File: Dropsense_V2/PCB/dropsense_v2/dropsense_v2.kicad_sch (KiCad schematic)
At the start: 28 parts, among them J1 Micro_SD_Card_Det_Hirose_DM3AT, J2 USB_B_Micro, J3 battery socket, SW1 SW_Push, SW2 SW_Push, U1 ESP32-S3-WROOM-1, U2 MPU-6050, U3 TP4056-42-ESOP8, U4 ME6211C10M5

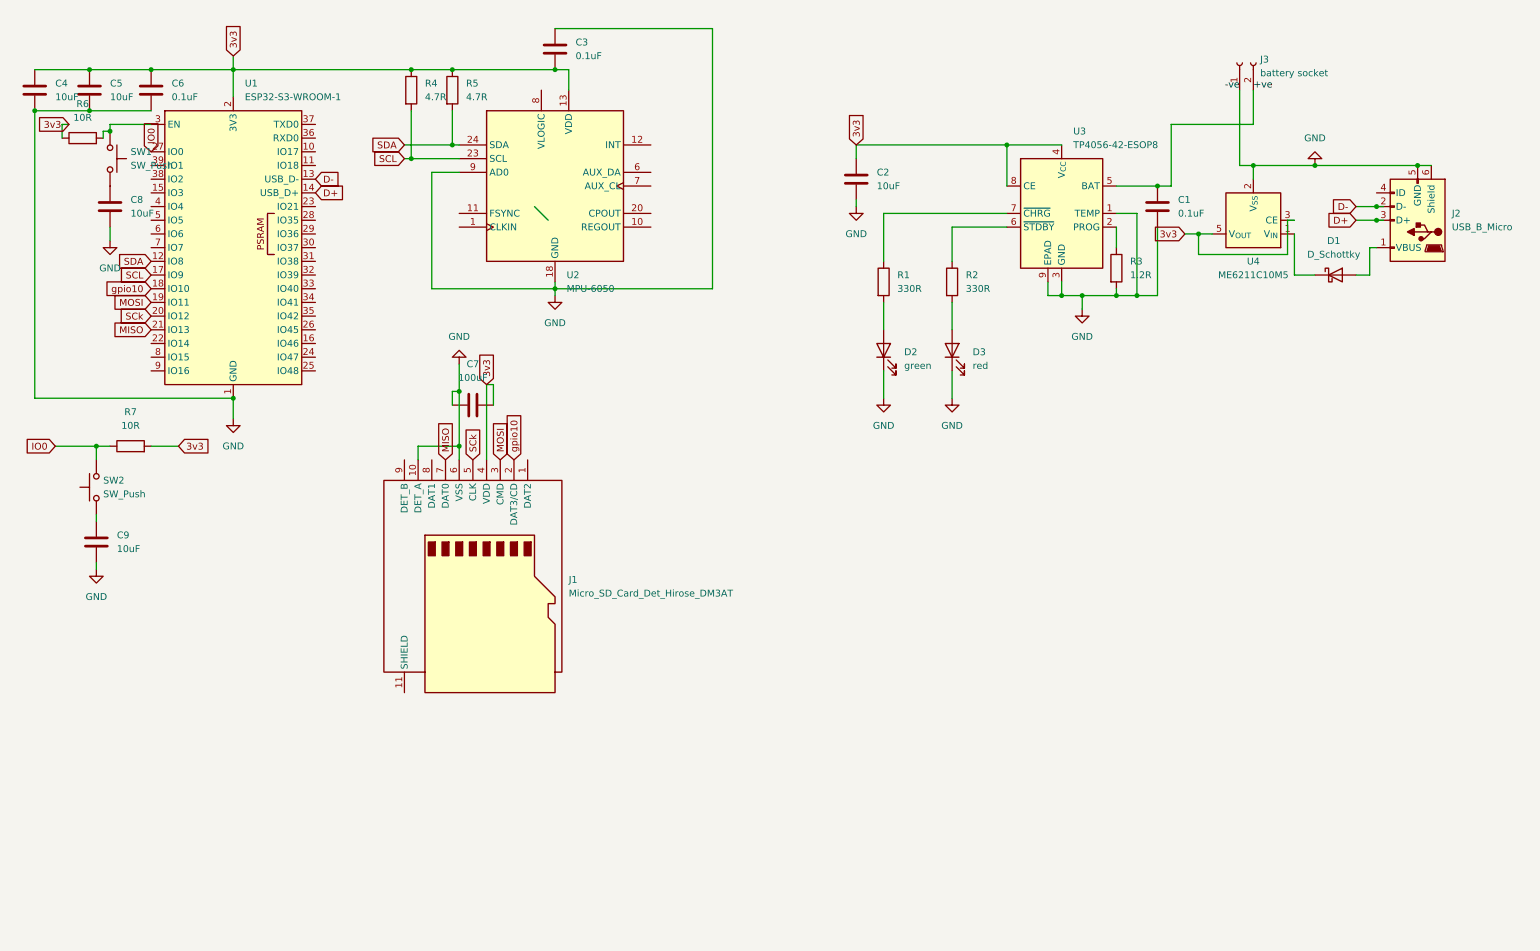
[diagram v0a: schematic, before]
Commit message: STARTED DROPSENSE V2!!!!!!
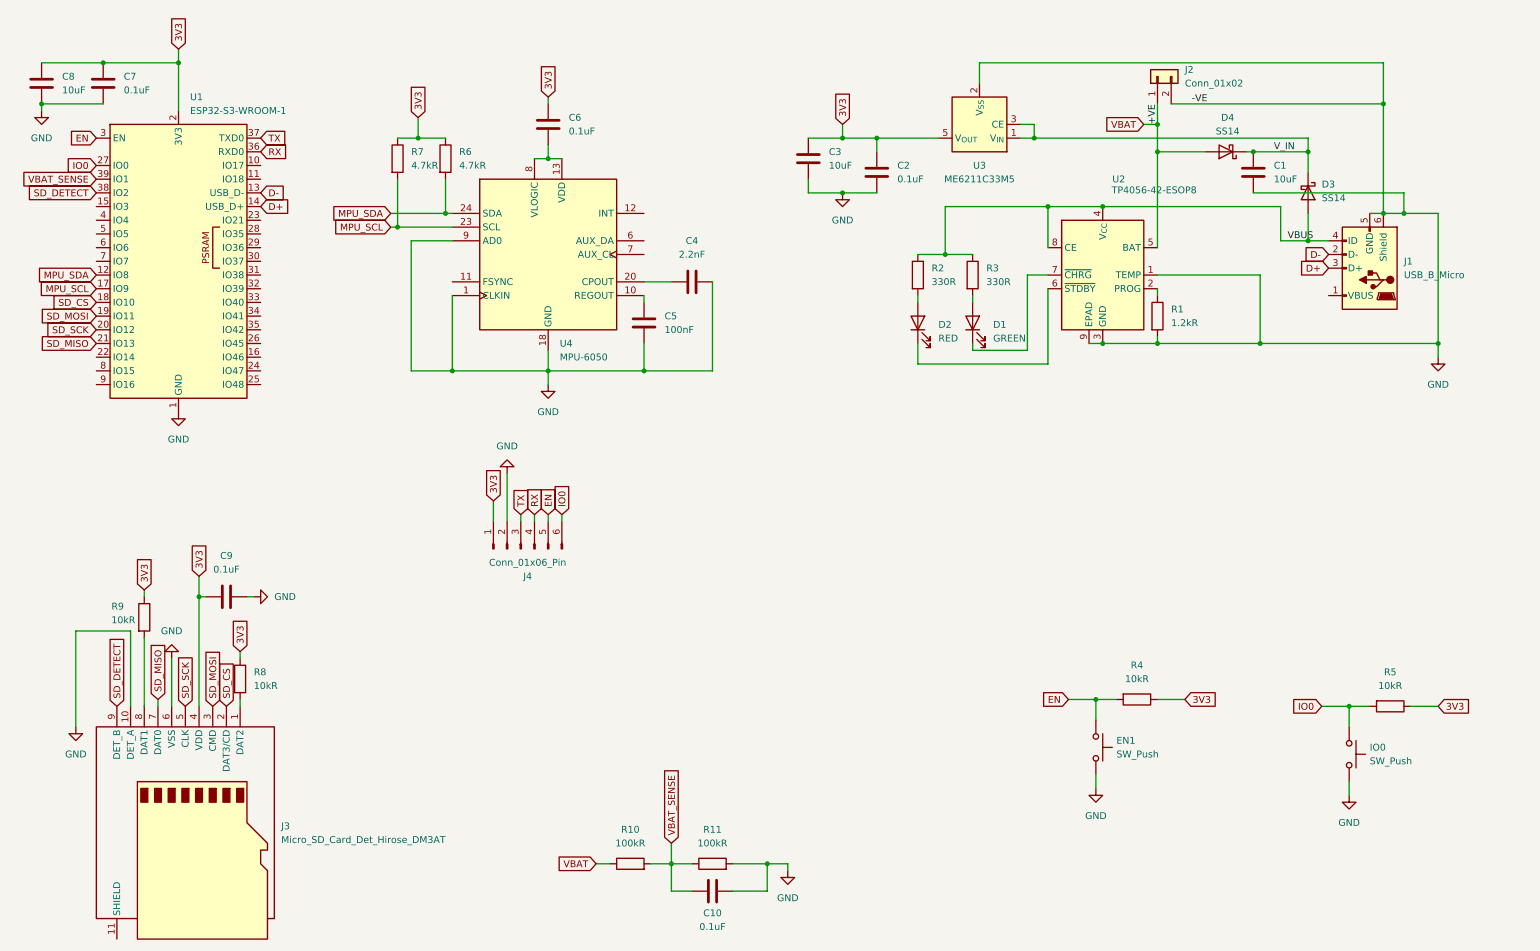
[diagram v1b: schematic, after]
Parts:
- removed D1: D_Schottky, Diode_SMD:D_0805_2012Metric, symbol Device:D_Schottky
- removed D3: red, LED_SMD:LED_0805_2012Metric, symbol Device:LED
- removed J1: Micro_SD_Card_Det_Hirose_DM3AT, Connector_Card:microSD_HC_Hirose_DM3AT-SF-PEJM5, symbol Connector:Micro_SD_Card_Det_Hirose_DM3AT
- removed J2: USB_B_Micro, Connector_USB:USB_Micro-B_Amphenol_10103594-0001LF_Horizontal, symbol Connector:USB_B_Micro
- removed J3: battery socket, Connector_JST:JST_PH_B2B-PH-K_1x02_P2.00mm_Vertical, symbol Connector:Conn_01x02_Socket
- removed SW1, SW2: SW_Push, Button_Switch_THT:SW_PUSH_6mm_H4.3mm, symbol Switch:SW_Push
- removed U2: MPU-6050, Sensor_Motion:InvenSense_QFN-24_4x4mm_P0.5mm, symbol Sensor_Motion:MPU-6050
- removed U3: TP4056-42-ESOP8, Package_SO:SOIC-8-1EP_3.9x4.9mm_P1.27mm_EP2.41x3.3mm_ThermalVias, symbol Battery_Management:TP4056-42-ESOP8
- removed U4: ME6211C10M5, Package_TO_SOT_SMD:SOT-23-5, symbol Regulator_Linear:ME6211C10M5
- added C10: 0.1uF, Capacitor_SMD:C_0805_2012Metric, symbol Device:C
- added D1: GREEN, LED_SMD:LED_0805_2012Metric, symbol Device:LED
- added D3, D4: SS14, Diode_SMD:D_SMA, symbol Diode:SS14
- added EN1, IO0: SW_Push, Button_Switch_SMD:SW_Push_1P1T-SH_NO_CK_KMR2xxG, symbol Switch:SW_Push
- added J1: USB_B_Micro, Connector_USB:USB_Micro-B_Molex-105017-0001, symbol Connector:USB_B_Micro
- added J2: Conn_01x02, Connector_JST:JST_XH_B2B-XH-A_1x02_P2.50mm_Vertical, symbol Connector_Generic:Conn_01x02
- added J3: Micro_SD_Card_Det_Hirose_DM3AT, Connector_Card:microSD_HC_Hirose_DM3AT-SF-PEJM5, symbol Connector:Micro_SD_Card_Det_Hirose_DM3AT
- added J4: Conn_01x06_Pin, Connector_PinHeader_2.54mm:PinHeader_1x06_P2.54mm_Vertical, symbol Connector:Conn_01x06_Pin
- added R10, R11: 100kR, Resistor_SMD:R_0805_2012Metric, symbol Device:R
- added R8, R9: 10kR, Resistor_SMD:R_0805_2012Metric, symbol Device:R
- added U2: TP4056-42-ESOP8, Package_SO:SOIC-8-1EP_3.9x4.9mm_P1.27mm_EP2.41x3.3mm_ThermalVias, symbol Battery_Management:TP4056-42-ESOP8
- added U3: ME6211C33M5, Package_TO_SOT_SMD:SOT-23-5, symbol Regulator_Linear:ME6211C33M5
- added U4: MPU-6050, Sensor_Motion:InvenSense_QFN-24_4x4mm_P0.5mm, symbol Sensor_Motion:MPU-6050
- C1, C3: value 0.1uF -> 10uF
- C2, C9: value 10uF -> 0.1uF
- C4: value 10uF -> 2.2nF
- C5: value 10uF -> 100nF
- C7: value 100uF -> 0.1uF
- D2: value green -> RED
- R1: value 330R -> 1.2kR
- R3: value 1.2R -> 330R
- R4, R5: value 4.7R -> 10kR
- R6, R7: value 10R -> 4.7kR
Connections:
- net D+: now also J1.3 (D+)
- net D-: now also J1.2 (D-)
- net GND: now also C3.2, C5.1, C7.2, R1.2, C10.2, EN1.2, IO0.2, J1.5 (GND), J1.6 (Shield), J2.2 (Pin_2), J3.10 (DET_A), J3.6 (VSS), J4.2 (Pin_2), R11.2, U2.1 (TEMP), U2.3 (GND), U2.9 (EPAD), U3.2 (V_{SS}), U4.1 (CLKIN), U4.18 (GND), U4.9 (AD0); no longer C3.1, C5.2, C6.2, C7.1, D2.1 (K), R3.2
- net IO0: now also R5.2, IO0.1, J4.6 (Pin_6); no longer R7.1
- net at R2.2: now also D2.2 (A)
- net 3V3: now reaches C9.1
- net 3V3: now also C2.1, C3.1, C6.1, C7.1, C8.1, R4.1, R5.1, R6.1, R7.1, U1.2 (3V3), J3.4 (VDD), J4.1 (Pin_1), R8.1, R9.1, U3.5 (V_{OUT})
- net EN: now reaches U1.3 (EN)
- net EN: now also R4.2, EN1.1, J4.5 (Pin_5); no longer R6.2
- net RX: now reaches U1.36 (RXD0)
- net RX: now also J4.4 (Pin_4)
- net TX: now reaches U1.37 (TXD0)
- net TX: now also J4.3 (Pin_3)
- net SD_DETECT: now reaches U1.38 (IO2)
- net SD_DETECT: now also J3.9 (DET_B)
- net VBAT_SENSE: now reaches U1.39 (IO1)
- net VBAT_SENSE: now also C10.1, R10.2, R11.1
- net VBUS: now reaches R2.1
- net VBUS: now also R3.1, D3.2 (A), J1.4 (ID), U2.4 (V_{CC}), U2.8 (CE)
- net at R1.1: now also U2.2 (PROG)
- net +ve renamed V_IN
- net V_IN: now also D3.1 (K), D4.1 (K), U3.1 (V_{IN}), U3.3 (CE)
- removed net 3v3: C2.1, C3.2, C4.1, C5.1, C6.1, C7.2, R4.1, R5.1, R6.1, R7.2, U1.2 (3V3)
- net MISO renamed SD_MISO
- net SD_MISO: now also J3.7 (DAT0)
- net MOSI renamed SD_MOSI
- net SD_MOSI: now also J3.3 (CMD)
- net SCL renamed MPU_SCL
- net MPU_SCL: now also R7.2, U4.23 (SCL); no longer R4.2
- net SCk renamed SD_SCK
- net SD_SCK: now also J3.5 (CLK)
- net SDA renamed MPU_SDA
- net MPU_SDA: now also R6.2, U4.24 (SDA); no longer R5.2
- net gpio10 renamed SD_CS
- net SD_CS: now also J3.2 (DAT3/CD)
- new net: D1.1 (K), U2.7 (~{CHRG})
- new net: D1.2 (A), R3.2
- new net: J3.8 (DAT1), R9.2
- new net: D2.1 (K), U2.6 (~{STDBY})
- new net: J3.1 (DAT2), R8.2
- new net: C5.2, U4.10 (REGOUT)
- new net: C6.2, U4.13 (VDD), U4.8 (VLOGIC)
- new net: C4.1, U4.20 (CPOUT)
- new net VBAT: D4.2 (A), J2.1 (Pin_1), R10.1, U2.5 (BAT)
